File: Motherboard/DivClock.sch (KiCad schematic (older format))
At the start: 26 parts, among them SW1 TURBO, SW2 FREEZE, U10 4081, U11 4081, U12 74LS32, U13 74LS14, U14 74LS77, U15 74LS257, U16 4069, U17 74LS32, U18 4081, U19 74HC74, U20 7402, U21 40106, U8 4069, U9 40106, Y1 18.432 MHz, Y2 32.768 MHz

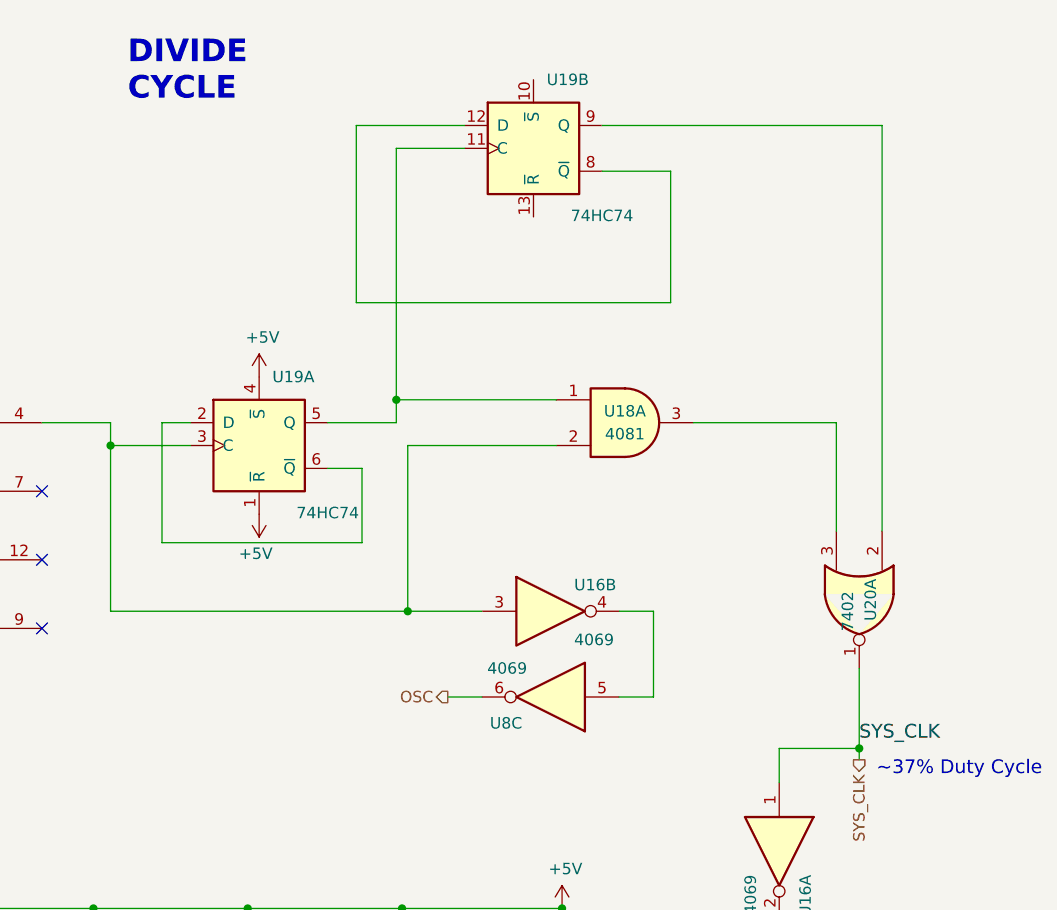
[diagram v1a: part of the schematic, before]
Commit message: Large sync
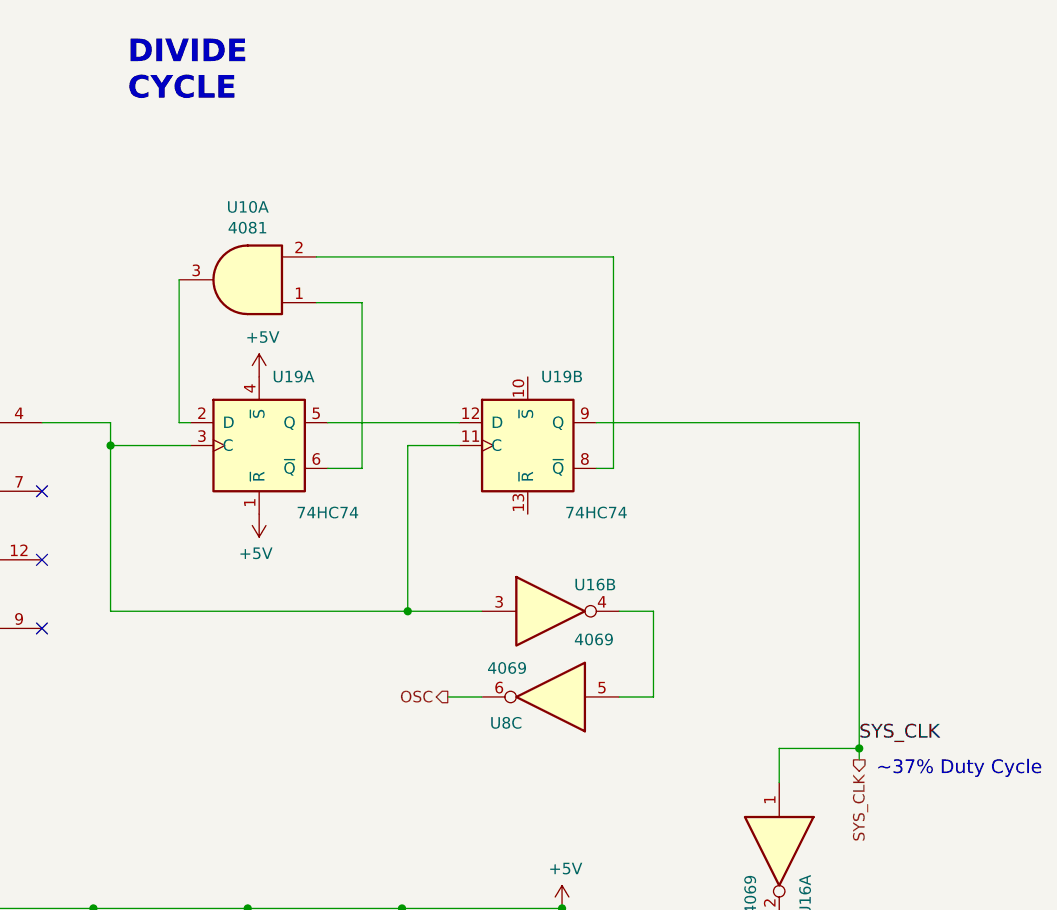
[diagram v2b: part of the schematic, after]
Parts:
- removed unit 1 of U18
- removed unit 1 of U20
- added unit 1 of U10
- U13: footprint (none) -> Housings_DIP:DIP-14_W7.62mm_Socket
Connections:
- net SYS_CLK: now also U19.9 (Q)
- net at U15.4 (Za), U16.3, U19.3 (C): now also U19.11 (C)
- net at U19.2 (D): now also U10.3; no longer U19.6 (~Q)
- net at U19.5 (Q): now also U19.12 (D); no longer U19.11 (C)
- net at U19.8 (~Q): now also U10.2; no longer U19.12 (D)
- new net: U10.1, U19.6 (~Q)
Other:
- moved on the sheet: U19B
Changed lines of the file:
@@
 L 74xx:74HC74 U19
 U 2 1 5BFDC06F
-P 8775 1225
-F 0 "U19" H 8925 1525 50  0000 C CNN
-F 1 "74HC74" H 9075 930 50  0000 C CNN
-F 2 "Housings_DIP:DIP-14_W7.62mm_Socket" H 8775 1225 50  0001 C CNN
-F 3 "" H 8775 1225 50  0001 C CNN
-	2    8775 1225
-	1    0    0    -1
-$EndComp
-$Comp
-L 4xxx:4081 U18
-U 1 1 5BFDE512
-P 9175 2425
-F 0 "U18" H 9175 2475 50  0000 C CNN
-F 1 "4081" H 9175 2375 50  0000 C CNN
-F 2 "Housings_DIP:DIP-14_W7.62mm_Socket" H 9175 2425 60  0001 C CNN
-F 3 "" H 9175 2425 60  0001 C CNN
-	1    9175 2425
-	1    0    0    -1
-$EndComp
-$Comp
-L 74xx:7402 U20
-U 1 1 5BFDF6A5
-P 10200 3200
-F 0 "U20" H 10200 3250 50  0000 C CNN
-F 1 "7402" H 10250 3150 50  0000 C CNN
-F 2 "Housings_DIP:DIP-14_W7.62mm_Socket" H 10200 3200 50  0001 C CNN
-F 3 "" H 10200 3200 50  0001 C CNN
-	1    10200 3200
-	0    1    1    0
+P 8750 2525
+F 0 "U19" H 8900 2825 50  0000 C CNN
+F 1 "74HC74" H 9050 2230 50  0000 C CNN
+F 2 "Housings_DIP:DIP-14_W7.62mm_Socket" H 8750 2525 50  0001 C CNN
+F 3 "" H 8750 2525 50  0001 C CNN
+	2    8750 2525
+	1    0    0    -1
 $EndComp
 Text Label 10200 3825 0    60   ~ 0
@@
 	3975 2475 5375 2475
 Wire Wire Line
-	9375 1900 8000 1900
-Wire Wire Line
-	8000 1900 8000 1125
-Wire Wire Line
 	6925 2525 6925 3250
 Wire Wire Line
@@
 	7875 2625 8025 2625
 Wire Wire Line
-	8025 2625 8025 2950
-Wire Wire Line
-	8025 2950 7150 2950
-Wire Wire Line
-	7150 2950 7150 2425
-Wire Wire Line
-	7150 2425 7275 2425
-Wire Wire Line
 	6925 2525 7275 2525
 Wire Wire Line
@@
 	-1   0    0    1
 $EndComp
-Wire Wire Line
-	7875 2425 8175 2425
-Wire Wire Line
-	8175 2425 8175 2325
-Connection ~ 8175 2325
-Wire Wire Line
-	8175 1225 8475 1225
-Wire Wire Line
-	8175 1225 8175 2325
-Wire Wire Line
-	8000 1125 8475 1125
-Wire Wire Line
-	9375 1325 9075 1325
-Wire Wire Line
-	9375 1325 9375 1900
-Wire Wire Line
-	9075 1125 10300 1125
-Wire Wire Line
-	8175 2325 8875 2325
-Wire Wire Line
-	8225 2525 8875 2525
-Wire Wire Line
-	9475 2425 10100 2425
-Wire Wire Line
-	10100 2425 10100 2900
-Wire Wire Line
-	10300 1125 10300 2900
-Wire Wire Line
-	10200 3500 10200 3850
 Wire Wire Line
 	9850 3850 9850 4000
@@
 F 0 "U13" V 4379 5805 50  0000 L CNN
 F 1 "74LS14" V 4470 5805 50  0000 L CNN
-F 2 "" H 4425 5625 50  0001 C CNN
+F 2 "Housings_DIP:DIP-14_W7.62mm_Socket" H 4425 5625 50  0001 C CNN
 F 3 "http://www.ti.com/lit/gpn/sn74LS14" H 4425 5625 50  0001 C CNN
 	1    4425 5625
 	0    1    1    0
 $EndComp
+Wire Wire Line
+	7875 2425 8450 2425
+Wire Wire Line
+	8450 2525 8225 2525
+$Comp
+L 4xxx:4081 U10
+U 1 1 5C493CC7
+P 7525 1800
+F 0 "U10" H 7525 1483 50  0000 C CNN
+F 1 "4081" H 7525 1574 50  0000 C CNN
+F 2 "Housings_DIP:DIP-14_W7.62mm_Socket" H 7525 1800 50  0001 C CNN
+F 3 "http://www.intersil.com/content/dam/Intersil/documents/cd40/cd4073bms-81bms-82bms.pdf" H 7525 1800 50  0001 C CNN
+	1    7525 1800
+	-1   0    0    1
+$EndComp
+Wire Wire Line
+	7225 1800 7225 2425
+Wire Wire Line
+	7225 2425 7275 2425
+Wire Wire Line
+	7825 1900 8025 1900
+Wire Wire Line
+	8025 1900 8025 2625
+Wire Wire Line
+	9050 2625 9125 2625
+Wire Wire Line
+	9125 2625 9125 1700
+Wire Wire Line
+	9125 1700 7825 1700
+Wire Wire Line
+	9050 2425 10200 2425
+Wire Wire Line
+	10200 2425 10200 3850
 $EndSCHEMATC
